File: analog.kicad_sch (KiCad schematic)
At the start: 39 parts, among them Q3 BSS138, U1 TL494, U4 NE5532, U5 INA180A2

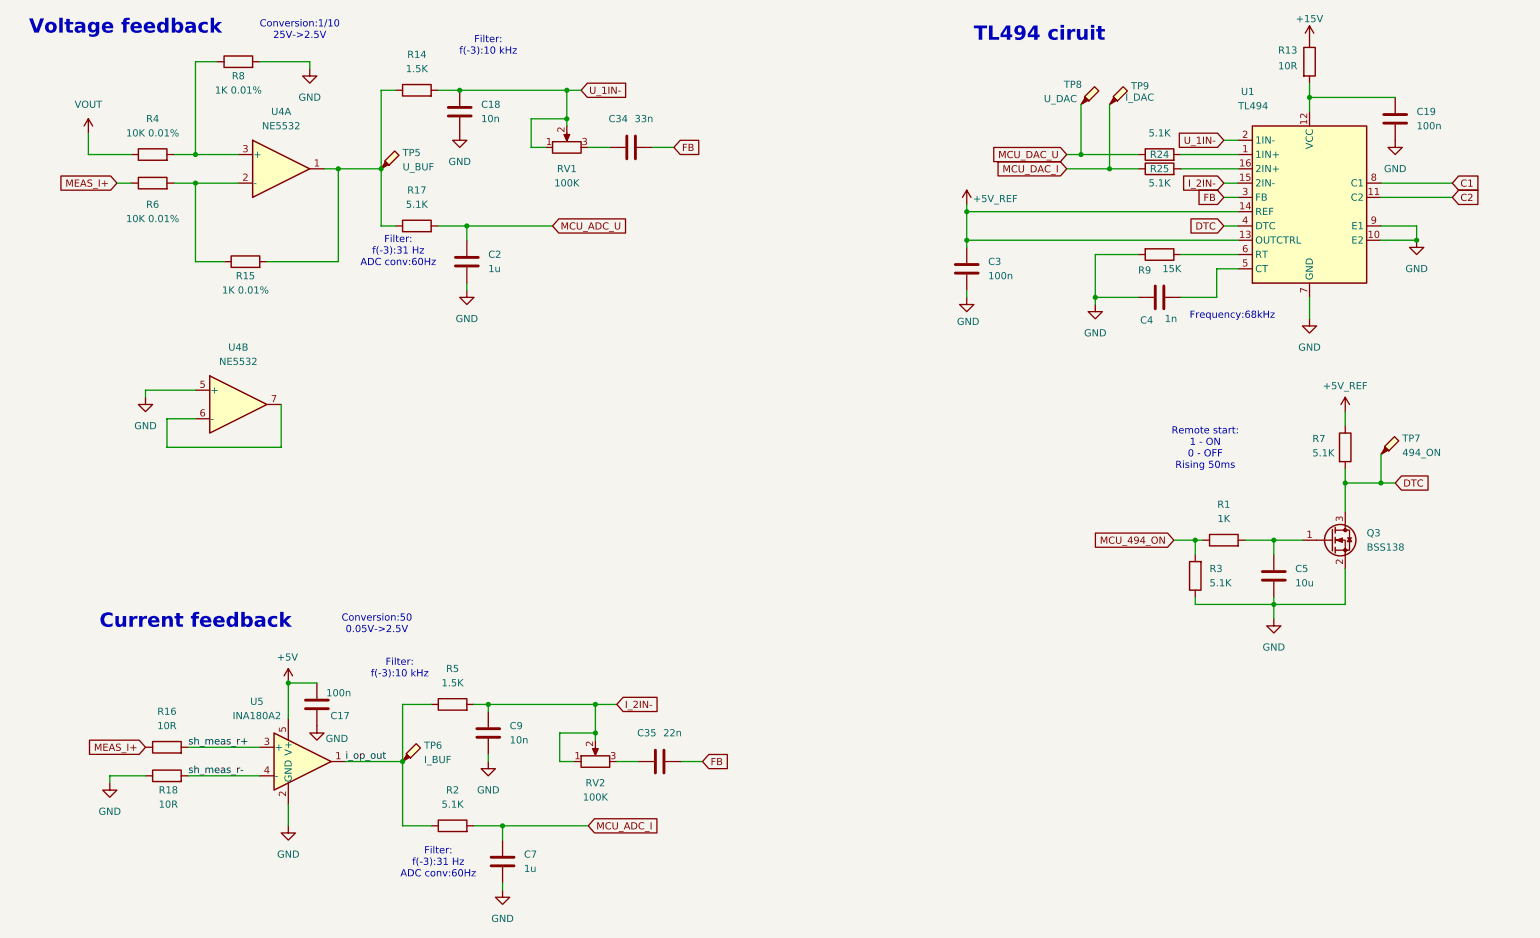
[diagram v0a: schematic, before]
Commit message: final location of the power,analog sections
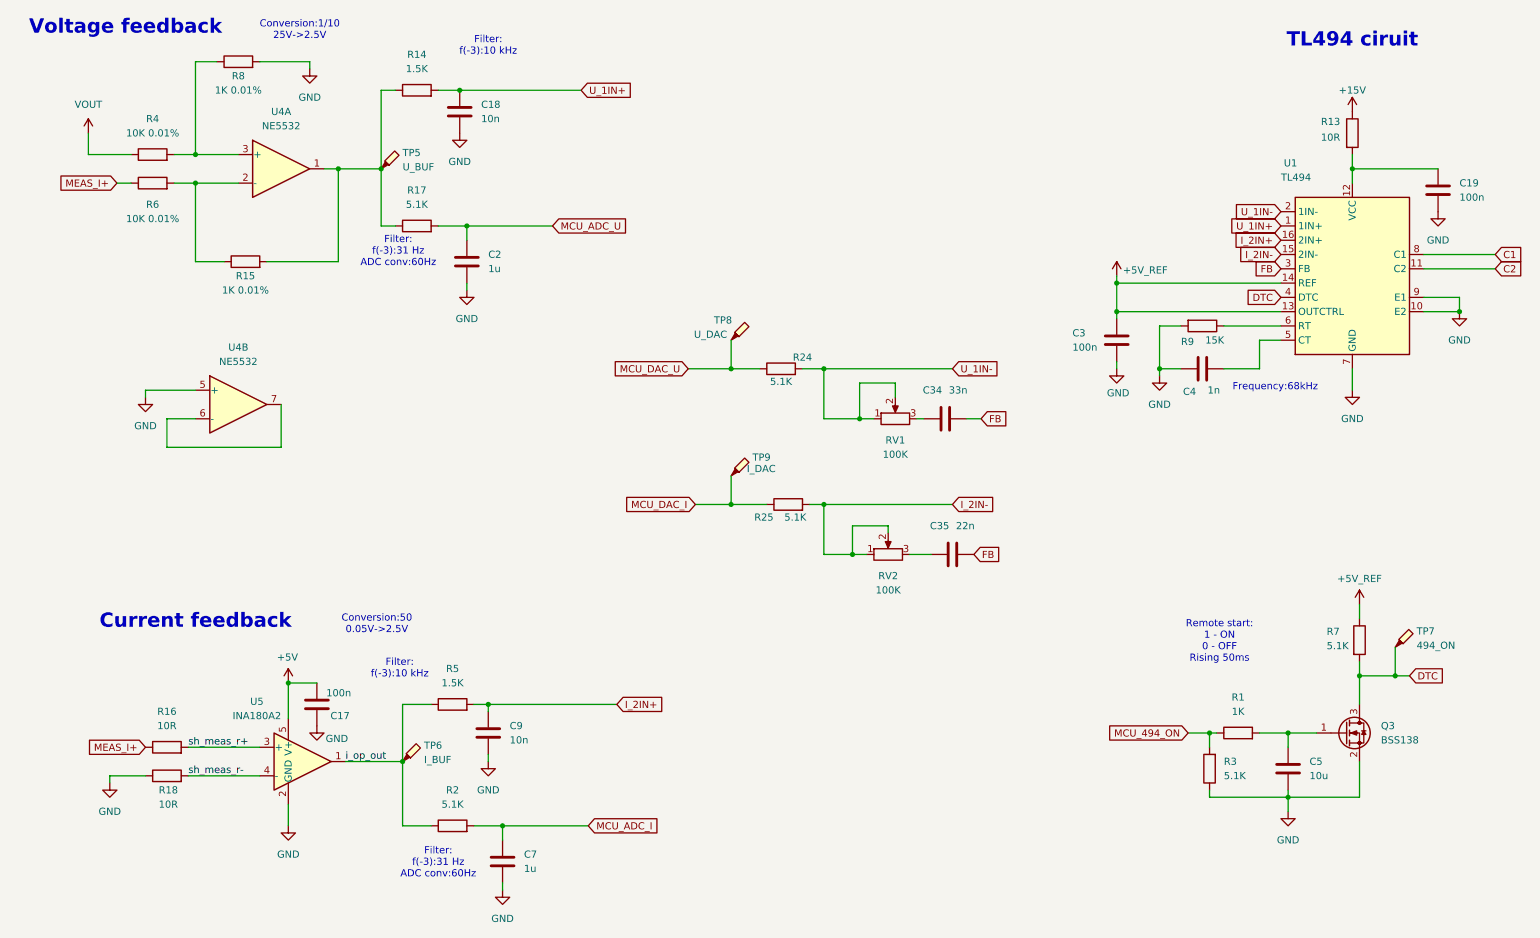
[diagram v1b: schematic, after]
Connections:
- net I_2IN-: now also R25.2; no longer C9.1, R5.2
- net U_1IN-: now also R24.2; no longer C18.1, R14.2
- net I_2IN+: now reaches U1.16 (2IN+)
- net I_2IN+: now also C9.1, R5.2; no longer R25.2
- net U_1IN+: now reaches U1.1 (1IN+)
- net U_1IN+: now also C18.1, R14.2; no longer R24.2
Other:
- moved on the sheet: C19, C3, C34, C35, C4, C5, Q3, R1, R13, R24, R25, R3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
